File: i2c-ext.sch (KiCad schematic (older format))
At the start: 5 parts, among them J1101 SMBUS, U1101 TCA9802

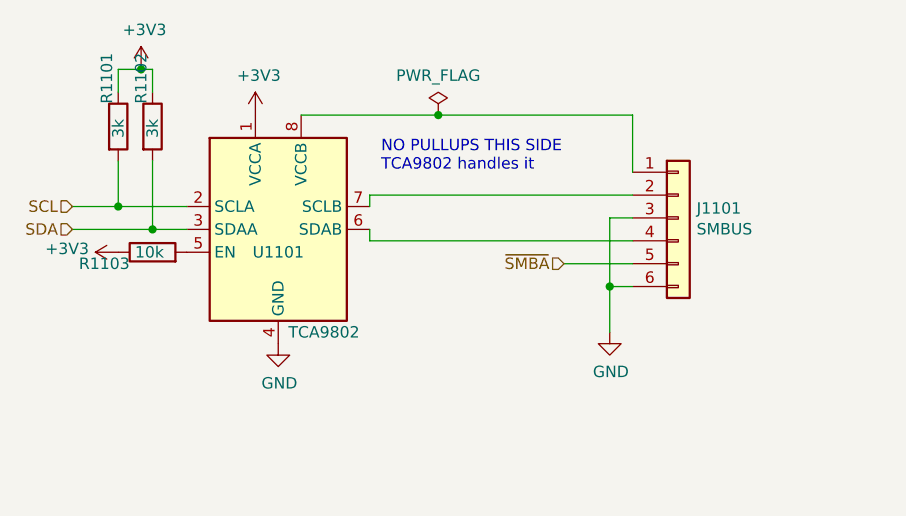
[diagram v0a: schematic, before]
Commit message: MB: switch buttons to cheap, readily available parts
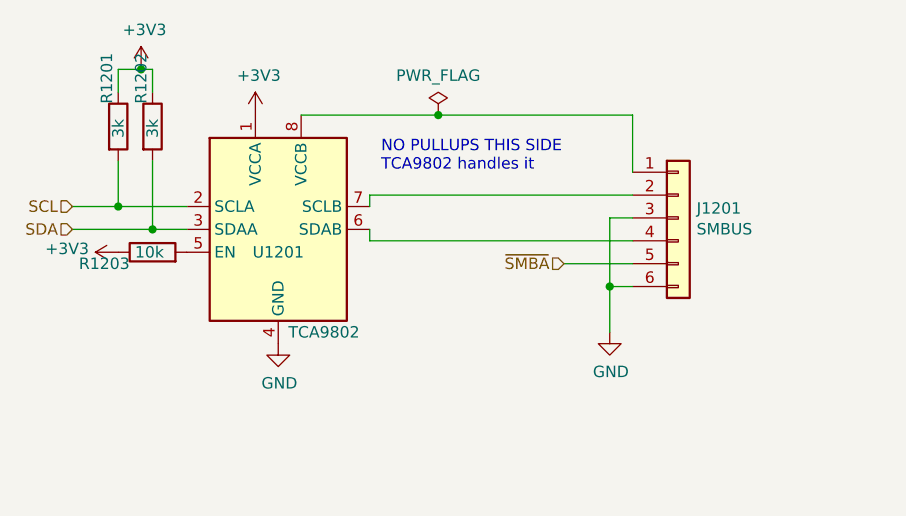
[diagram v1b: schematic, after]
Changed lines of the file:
@@
 $Descr A4 11693 8268
 encoding utf-8
-Sheet 11 15
+Sheet 12 15
 Title "Offboard I2C connector (one bus)"
 Date ""
@@
 AR Path="/5F2FE5B6/5F2F1DD6" Ref="U1201"  Part="1"
 AR Path="/5F3042B8/5F2F1DD6" Ref="U1301"  Part="1"
-F 0 "U1101" H 5600 3550 50  0000 C CNN
+F 0 "U1201" H 5600 3550 50  0000 C CNN
 F 1 "TCA9802" H 5800 3200 50  0000 C CNN
 F 2 "Package_SO:VSSOP-8_3.0x3.0mm_P0.65mm" H 6500 3200 50  0001 C CNN
@@
 AR Path="/5F2FE5B6/5F2F21C9" Ref="#PWR01203"  Part="1"
 AR Path="/5F3042B8/5F2F21C9" Ref="#PWR01303"  Part="1"
-F 0 "#PWR01103" H 5500 3000 50  0001 C CNN
+F 0 "#PWR01303" H 5500 3000 50  0001 C CNN
 F 1 "+3V3" H 5515 3323 50  0000 C CNN
 F 2 "" H 5500 3150 50  0001 C CNN
@@
 AR Path="/5F2FE5B6/5F2F2367" Ref="#PWR01204"  Part="1"
 AR Path="/5F3042B8/5F2F2367" Ref="#PWR01304"  Part="1"
-F 0 "#PWR01104" H 5600 3900 50  0001 C CNN
+F 0 "#PWR01304" H 5600 3900 50  0001 C CNN
 F 1 "GND" H 5605 3977 50  0000 C CNN
 F 2 "" H 5600 4150 50  0001 C CNN
@@
 AR Path="/5F2FE5B6/5F2F26BC" Ref="J1201"  Part="1"
 AR Path="/5F3042B8/5F2F26BC" Ref="J1301"  Part="1"
-F 0 "J1101" H 7430 3642 50  0000 L CNN
+F 0 "J1201" H 7430 3642 50  0000 L CNN
 F 1 "SMBUS" H 7430 3551 50  0000 L CNN
 F 2 "molex-sl:SL_1x06_Vertical_SMD" H 7350 3600 50  0001 C CNN
@@
 AR Path="/5F2FE5B6/5F2F3249" Ref="#PWR01205"  Part="1"
 AR Path="/5F3042B8/5F2F3249" Ref="#PWR01305"  Part="1"
-F 0 "#PWR01105" H 7050 3850 50  0001 C CNN
+F 0 "#PWR01305" H 7050 3850 50  0001 C CNN
 F 1 "GND" H 7055 3927 50  0000 C CNN
 F 2 "" H 7050 4100 50  0001 C CNN
@@
 AR Path="/5F2FE5B6/5F2F4AED" Ref="R1201"  Part="1"
 AR Path="/5F3042B8/5F2F4AED" Ref="R1301"  Part="1"
-F 0 "R1101" V 4850 3300 50  0000 L CNN
+F 0 "R1201" V 4850 3300 50  0000 L CNN
 F 1 "3k" V 4900 3150 50  0000 L CNN
 F 2 "Resistor_SMD:R_0603_1608Metric" V 4830 3200 50  0001 C CNN
@@
 AR Path="/5F2FE5B6/5F2F511D" Ref="R1202"  Part="1"
 AR Path="/5F3042B8/5F2F511D" Ref="R1302"  Part="1"
-F 0 "R1102" V 5000 3300 50  0000 L CNN
+F 0 "R1202" V 5000 3300 50  0000 L CNN
 F 1 "3k" V 5050 3150 50  0000 L CNN
 F 2 "Resistor_SMD:R_0603_1608Metric" V 4980 3200 50  0001 C CNN
@@
 AR Path="/5F2FE5B6/5F2F5A4A" Ref="#PWR01202"  Part="1"
 AR Path="/5F3042B8/5F2F5A4A" Ref="#PWR01302"  Part="1"
-F 0 "#PWR01102" H 5000 2800 50  0001 C CNN
+F 0 "#PWR01302" H 5000 2800 50  0001 C CNN
 F 1 "+3V3" H 5015 3123 50  0000 C CNN
 F 2 "" H 5000 2950 50  0001 C CNN
@@
 AR Path="/5F2FE5B6/600BC5DC" Ref="R1203"  Part="1"
 AR Path="/5F3042B8/600BC5DC" Ref="R1303"  Part="1"
-F 0 "R1103" V 5000 3850 50  0000 L CNN
+F 0 "R1203" V 5000 3850 50  0000 L CNN
 F 1 "10k" V 5050 3700 50  0000 L CNN
 F 2 "Resistor_SMD:R_0603_1608Metric" V 4980 3750 50  0001 C CNN
@@
 AR Path="/5F2FE5B6/600BD49C" Ref="#PWR01201"  Part="1"
 AR Path="/5F3042B8/600BD49C" Ref="#PWR01301"  Part="1"
-F 0 "#PWR01101" H 4900 3600 50  0001 C CNN
+F 0 "#PWR01301" H 4900 3600 50  0001 C CNN
 F 1 "+3V3" V 4915 3878 50  0000 L CNN
 F 2 "" H 4900 3750 50  0001 C CNN
@@
 AR Path="/5F2FE5B6/60108223" Ref="#FLG01201"  Part="1"
 AR Path="/5F3042B8/60108223" Ref="#FLG01301"  Part="1"
-F 0 "#FLG01101" H 6300 3225 50  0001 C CNN
+F 0 "#FLG01301" H 6300 3225 50  0001 C CNN
 F 1 "PWR_FLAG" H 6300 3323 50  0000 C CNN
 F 2 "" H 6300 3150 50  0001 C CNN

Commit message: MB: annotate everything with mfg/MPN
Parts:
- J1101: Mfg (none) -> Molex; Mfg Part Num (none) -> 0740991006
- R1101, R1102, R1103: Mfg Part Num (none) -> generic
- U1101: Mfg (none) -> Texas Instruments; Mfg Part Num (none) -> TCA9802
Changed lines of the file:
@@
 F 2 "Package_SO:VSSOP-8_3.0x3.0mm_P0.65mm" H 6500 3200 50  0001 C CNN
 F 3 "http://www.ti.com/lit/ds/symlink/tca9802.pdf" H 5300 4100 50  0001 C CNN
+F 4 "Texas Instruments" H 5600 3650 50  0001 C CNN "Mfg"
+F 5 "TCA9802" H 5600 3650 50  0001 C CNN "Mfg Part Num"
 	1    5600 3650
 	1    0    0    -1
@@
 F 2 "molex-sl:SL_1x06_Vertical_SMD" H 7350 3600 50  0001 C CNN
 F 3 "~" H 7350 3600 50  0001 C CNN
+F 4 "Molex" H 7350 3600 50  0001 C CNN "Mfg"
+F 5 "0740991006" H 7350 3600 50  0001 C CNN "Mfg Part Num"
 	1    7350 3600
 	1    0    0    -1
@@
 F 2 "Resistor_SMD:R_0603_1608Metric" V 4830 3200 50  0001 C CNN
 F 3 "~" H 4900 3200 50  0001 C CNN
+F 4 "generic" H 4900 3200 50  0001 C CNN "Mfg Part Num"
 	1    4900 3200
 	1    0    0    -1
@@
 F 2 "Resistor_SMD:R_0603_1608Metric" V 4980 3200 50  0001 C CNN
 F 3 "~" H 5050 3200 50  0001 C CNN
+F 4 "generic" H 5050 3200 50  0001 C CNN "Mfg Part Num"
 	1    5050 3200
 	1    0    0    -1
@@
 F 2 "Resistor_SMD:R_0603_1608Metric" V 4980 3750 50  0001 C CNN
 F 3 "~" H 5050 3750 50  0001 C CNN
+F 4 "generic" H 5050 3750 50  0001 C CNN "Mfg Part Num"
 	1    5050 3750
 	0    -1   -1   0

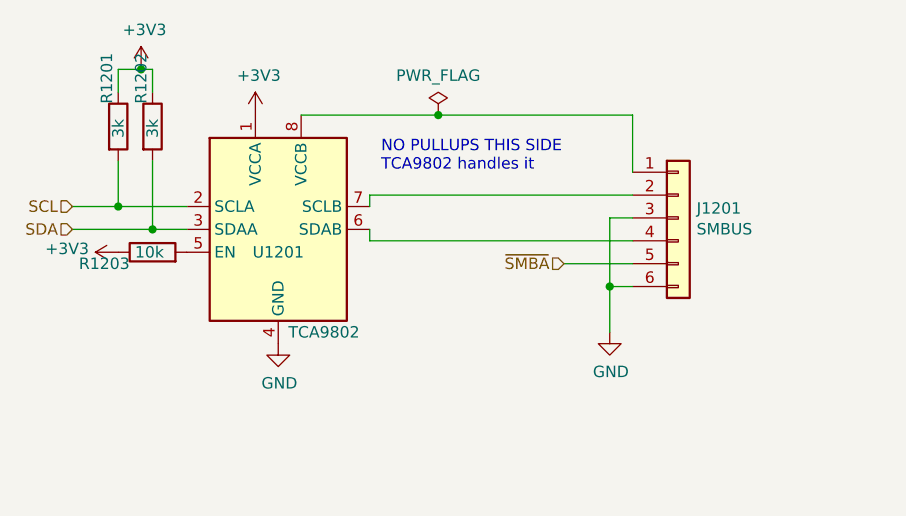
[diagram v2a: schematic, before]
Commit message: MB: assign single resistors
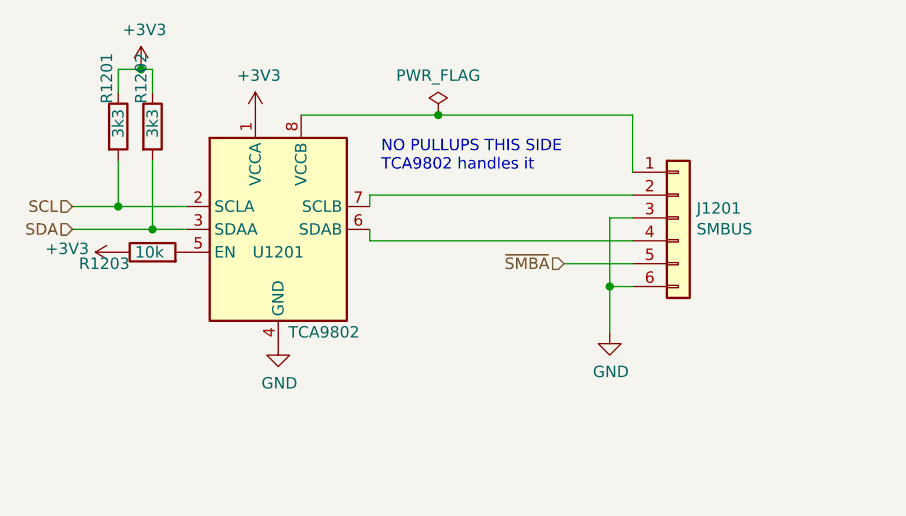
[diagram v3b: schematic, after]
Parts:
- R1101, R1102: value 3k -> 3k3; Mfg (none) -> Bourns; Mfg Part Num generic -> CR0603-JW-332ELF
- R1103: Mfg (none) -> Bourns; Mfg Part Num generic -> CR0603-JW-103ELF
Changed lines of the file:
@@
 AR Path="/5F3042B8/5F2F4AED" Ref="R1301"  Part="1"
 F 0 "R1201" V 4850 3300 50  0000 L CNN
-F 1 "3k" V 4900 3150 50  0000 L CNN
+F 1 "3k3" V 4900 3150 50  0000 L CNN
 F 2 "Resistor_SMD:R_0603_1608Metric" V 4830 3200 50  0001 C CNN
 F 3 "~" H 4900 3200 50  0001 C CNN
-F 4 "generic" H 4900 3200 50  0001 C CNN "Mfg Part Num"
+F 4 "CR0603-JW-332ELF" H 4900 3200 50  0001 C CNN "Mfg Part Num"
+F 5 "Bourns" H 4900 3200 50  0001 C CNN "Mfg"
 	1    4900 3200
 	1    0    0    -1
@@
 AR Path="/5F3042B8/5F2F511D" Ref="R1302"  Part="1"
 F 0 "R1202" V 5000 3300 50  0000 L CNN
-F 1 "3k" V 5050 3150 50  0000 L CNN
+F 1 "3k3" V 5050 3150 50  0000 L CNN
 F 2 "Resistor_SMD:R_0603_1608Metric" V 4980 3200 50  0001 C CNN
 F 3 "~" H 5050 3200 50  0001 C CNN
-F 4 "generic" H 5050 3200 50  0001 C CNN "Mfg Part Num"
+F 4 "CR0603-JW-332ELF" H 5050 3200 50  0001 C CNN "Mfg Part Num"
+F 5 "Bourns" H 5050 3200 50  0001 C CNN "Mfg"
 	1    5050 3200
 	1    0    0    -1
@@
 F 2 "Resistor_SMD:R_0603_1608Metric" V 4980 3750 50  0001 C CNN
 F 3 "~" H 5050 3750 50  0001 C CNN
-F 4 "generic" H 5050 3750 50  0001 C CNN "Mfg Part Num"
+F 4 "CR0603-JW-103ELF" H 5050 3750 50  0001 C CNN "Mfg Part Num"
+F 5 "Bourns" H 5050 3750 50  0001 C CNN "Mfg"
 	1    5050 3750
 	0    -1   -1   0

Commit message: MB: assign resistor networks
...and replace the x5 networks with discretes because they don't exist.
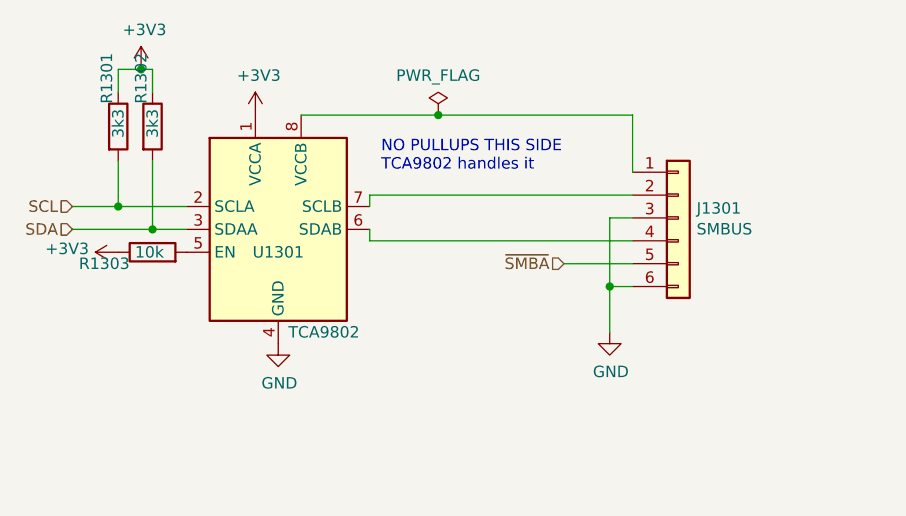
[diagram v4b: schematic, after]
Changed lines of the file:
@@
 AR Path="/5F2FE5B6/5F2F1DD6" Ref="U1201"  Part="1"
 AR Path="/5F3042B8/5F2F1DD6" Ref="U1301"  Part="1"
-F 0 "U1201" H 5600 3550 50  0000 C CNN
+F 0 "U1301" H 5600 3550 50  0000 C CNN
 F 1 "TCA9802" H 5800 3200 50  0000 C CNN
 F 2 "Package_SO:VSSOP-8_3.0x3.0mm_P0.65mm" H 6500 3200 50  0001 C CNN
@@
 AR Path="/5F2FE5B6/5F2F26BC" Ref="J1201"  Part="1"
 AR Path="/5F3042B8/5F2F26BC" Ref="J1301"  Part="1"
-F 0 "J1201" H 7430 3642 50  0000 L CNN
+F 0 "J1301" H 7430 3642 50  0000 L CNN
 F 1 "SMBUS" H 7430 3551 50  0000 L CNN
 F 2 "molex-sl:SL_1x06_Vertical_SMD" H 7350 3600 50  0001 C CNN
@@
 AR Path="/5F2FE5B6/5F2F4AED" Ref="R1201"  Part="1"
 AR Path="/5F3042B8/5F2F4AED" Ref="R1301"  Part="1"
-F 0 "R1201" V 4850 3300 50  0000 L CNN
+F 0 "R1301" V 4850 3300 50  0000 L CNN
 F 1 "3k3" V 4900 3150 50  0000 L CNN
 F 2 "Resistor_SMD:R_0603_1608Metric" V 4830 3200 50  0001 C CNN
@@
 AR Path="/5F2FE5B6/5F2F511D" Ref="R1202"  Part="1"
 AR Path="/5F3042B8/5F2F511D" Ref="R1302"  Part="1"
-F 0 "R1202" V 5000 3300 50  0000 L CNN
+F 0 "R1302" V 5000 3300 50  0000 L CNN
 F 1 "3k3" V 5050 3150 50  0000 L CNN
 F 2 "Resistor_SMD:R_0603_1608Metric" V 4980 3200 50  0001 C CNN
@@
 AR Path="/5F2FE5B6/600BC5DC" Ref="R1203"  Part="1"
 AR Path="/5F3042B8/600BC5DC" Ref="R1303"  Part="1"
-F 0 "R1203" V 5000 3850 50  0000 L CNN
+F 0 "R1303" V 5000 3850 50  0000 L CNN
 F 1 "10k" V 5050 3700 50  0000 L CNN
 F 2 "Resistor_SMD:R_0603_1608Metric" V 4980 3750 50  0001 C CNN

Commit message: MB: improve 3v3 and INA219 routing.
Per review comments from Mark.
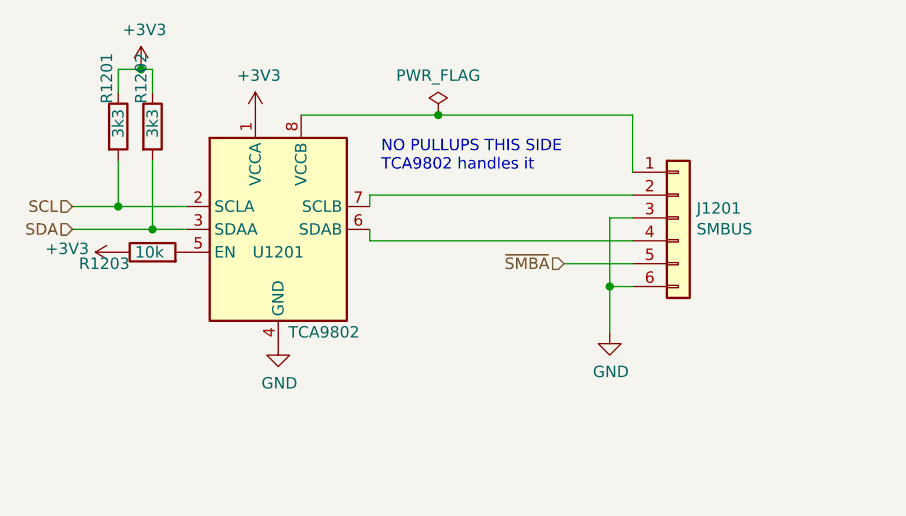
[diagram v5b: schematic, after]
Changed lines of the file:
@@
 AR Path="/5F2FE5B6/5F2F1DD6" Ref="U1201"  Part="1"
 AR Path="/5F3042B8/5F2F1DD6" Ref="U1301"  Part="1"
-F 0 "U1301" H 5600 3550 50  0000 C CNN
+F 0 "U1201" H 5600 3550 50  0000 C CNN
 F 1 "TCA9802" H 5800 3200 50  0000 C CNN
 F 2 "Package_SO:VSSOP-8_3.0x3.0mm_P0.65mm" H 6500 3200 50  0001 C CNN
@@
 AR Path="/5F2FE5B6/5F2F21C9" Ref="#PWR01203"  Part="1"
 AR Path="/5F3042B8/5F2F21C9" Ref="#PWR01303"  Part="1"
-F 0 "#PWR01303" H 5500 3000 50  0001 C CNN
+F 0 "#PWR01203" H 5500 3000 50  0001 C CNN
 F 1 "+3V3" H 5515 3323 50  0000 C CNN
 F 2 "" H 5500 3150 50  0001 C CNN
@@
 AR Path="/5F2FE5B6/5F2F2367" Ref="#PWR01204"  Part="1"
 AR Path="/5F3042B8/5F2F2367" Ref="#PWR01304"  Part="1"
-F 0 "#PWR01304" H 5600 3900 50  0001 C CNN
+F 0 "#PWR01204" H 5600 3900 50  0001 C CNN
 F 1 "GND" H 5605 3977 50  0000 C CNN
 F 2 "" H 5600 4150 50  0001 C CNN
@@
 AR Path="/5F2FE5B6/5F2F26BC" Ref="J1201"  Part="1"
 AR Path="/5F3042B8/5F2F26BC" Ref="J1301"  Part="1"
-F 0 "J1301" H 7430 3642 50  0000 L CNN
+F 0 "J1201" H 7430 3642 50  0000 L CNN
 F 1 "SMBUS" H 7430 3551 50  0000 L CNN
 F 2 "molex-sl:SL_1x06_Vertical_SMD" H 7350 3600 50  0001 C CNN
@@
 AR Path="/5F2FE5B6/5F2F3249" Ref="#PWR01205"  Part="1"
 AR Path="/5F3042B8/5F2F3249" Ref="#PWR01305"  Part="1"
-F 0 "#PWR01305" H 7050 3850 50  0001 C CNN
+F 0 "#PWR01205" H 7050 3850 50  0001 C CNN
 F 1 "GND" H 7055 3927 50  0000 C CNN
 F 2 "" H 7050 4100 50  0001 C CNN
@@
 AR Path="/5F2FE5B6/5F2F4AED" Ref="R1201"  Part="1"
 AR Path="/5F3042B8/5F2F4AED" Ref="R1301"  Part="1"
-F 0 "R1301" V 4850 3300 50  0000 L CNN
+F 0 "R1201" V 4850 3300 50  0000 L CNN
 F 1 "3k3" V 4900 3150 50  0000 L CNN
 F 2 "Resistor_SMD:R_0603_1608Metric" V 4830 3200 50  0001 C CNN
@@
 AR Path="/5F2FE5B6/5F2F511D" Ref="R1202"  Part="1"
 AR Path="/5F3042B8/5F2F511D" Ref="R1302"  Part="1"
-F 0 "R1302" V 5000 3300 50  0000 L CNN
+F 0 "R1202" V 5000 3300 50  0000 L CNN
 F 1 "3k3" V 5050 3150 50  0000 L CNN
 F 2 "Resistor_SMD:R_0603_1608Metric" V 4980 3200 50  0001 C CNN
@@
 AR Path="/5F2FE5B6/5F2F5A4A" Ref="#PWR01202"  Part="1"
 AR Path="/5F3042B8/5F2F5A4A" Ref="#PWR01302"  Part="1"
-F 0 "#PWR01302" H 5000 2800 50  0001 C CNN
+F 0 "#PWR01202" H 5000 2800 50  0001 C CNN
 F 1 "+3V3" H 5015 3123 50  0000 C CNN
 F 2 "" H 5000 2950 50  0001 C CNN
@@
 AR Path="/5F2FE5B6/600BC5DC" Ref="R1203"  Part="1"
 AR Path="/5F3042B8/600BC5DC" Ref="R1303"  Part="1"
-F 0 "R1303" V 5000 3850 50  0000 L CNN
+F 0 "R1203" V 5000 3850 50  0000 L CNN
 F 1 "10k" V 5050 3700 50  0000 L CNN
 F 2 "Resistor_SMD:R_0603_1608Metric" V 4980 3750 50  0001 C CNN
@@
 AR Path="/5F2FE5B6/600BD49C" Ref="#PWR01201"  Part="1"
 AR Path="/5F3042B8/600BD49C" Ref="#PWR01301"  Part="1"
-F 0 "#PWR01301" H 4900 3600 50  0001 C CNN
+F 0 "#PWR01201" H 4900 3600 50  0001 C CNN
 F 1 "+3V3" V 4915 3878 50  0000 L CNN
 F 2 "" H 4900 3750 50  0001 C CNN
@@
 AR Path="/5F2FE5B6/60108223" Ref="#FLG01201"  Part="1"
 AR Path="/5F3042B8/60108223" Ref="#FLG01301"  Part="1"
-F 0 "#FLG01301" H 6300 3225 50  0001 C CNN
+F 0 "#FLG01201" H 6300 3225 50  0001 C CNN
 F 1 "PWR_FLAG" H 6300 3323 50  0000 C CNN
 F 2 "" H 6300 3150 50  0001 C CNN
